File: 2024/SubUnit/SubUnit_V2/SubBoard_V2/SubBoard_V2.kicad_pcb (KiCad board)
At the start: 2 copper layers, 66.8 x 58 mm, 28 parts, among them J1 Conn_01x02_Socket, J10 Conn_01x02_Socket, J11 Conn_01x03_Socket, J12 Conn_01x02_Socket, J13 Conn_01x02_Socket, J14 Conn_01x05_Socket, J15 Conn_01x05_Socket, J16 Conn_01x02_Socket, J18 Conn_01x07_Socket, J19 Conn_01x07_Socket, J2 Conn_01x02_Socket, J3 Conn_01x02_Socket, J4 Conn_01x02_Socket, J5 Conn_01x02_Socket, J6 Conn_01x02_Socket, J7 Conn_01x02_Socket, J8 Conn_01x02_Socket, J9 Conn_01x02_Socket

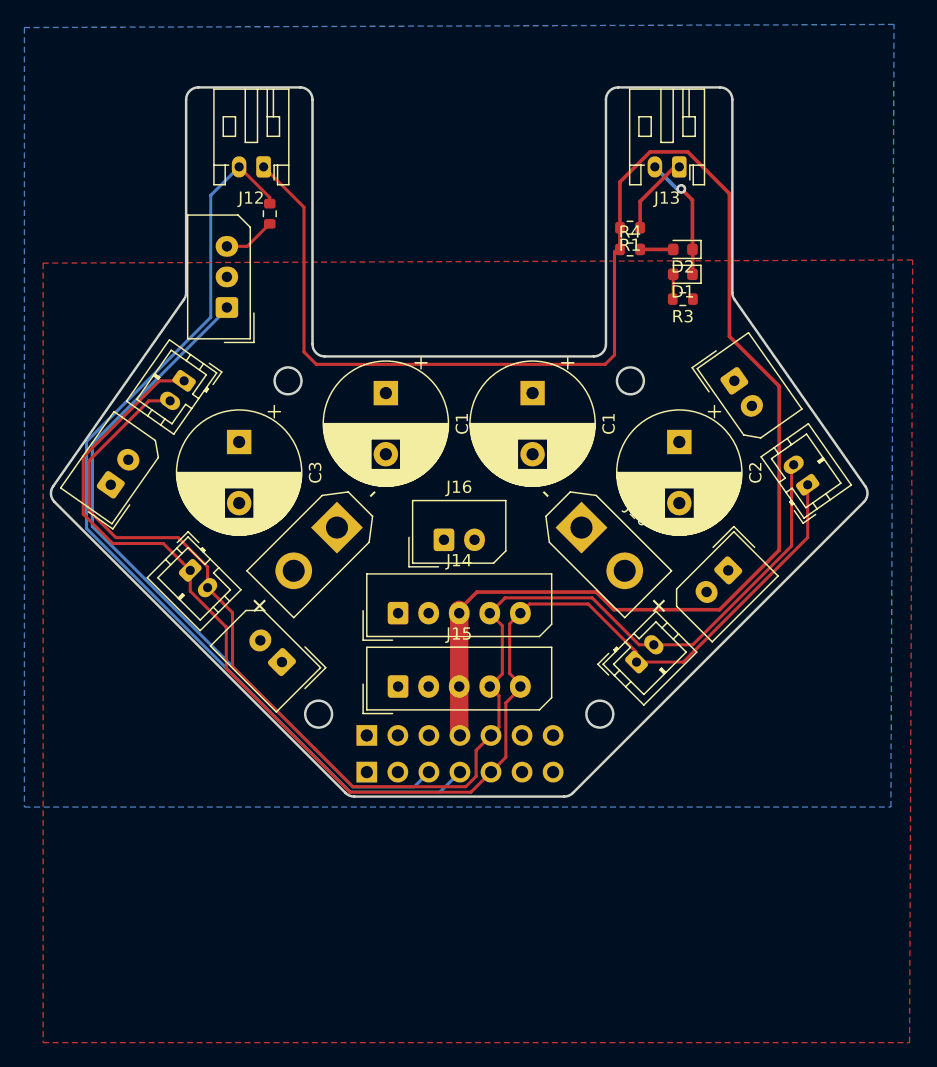
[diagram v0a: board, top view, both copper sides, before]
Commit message: 完成
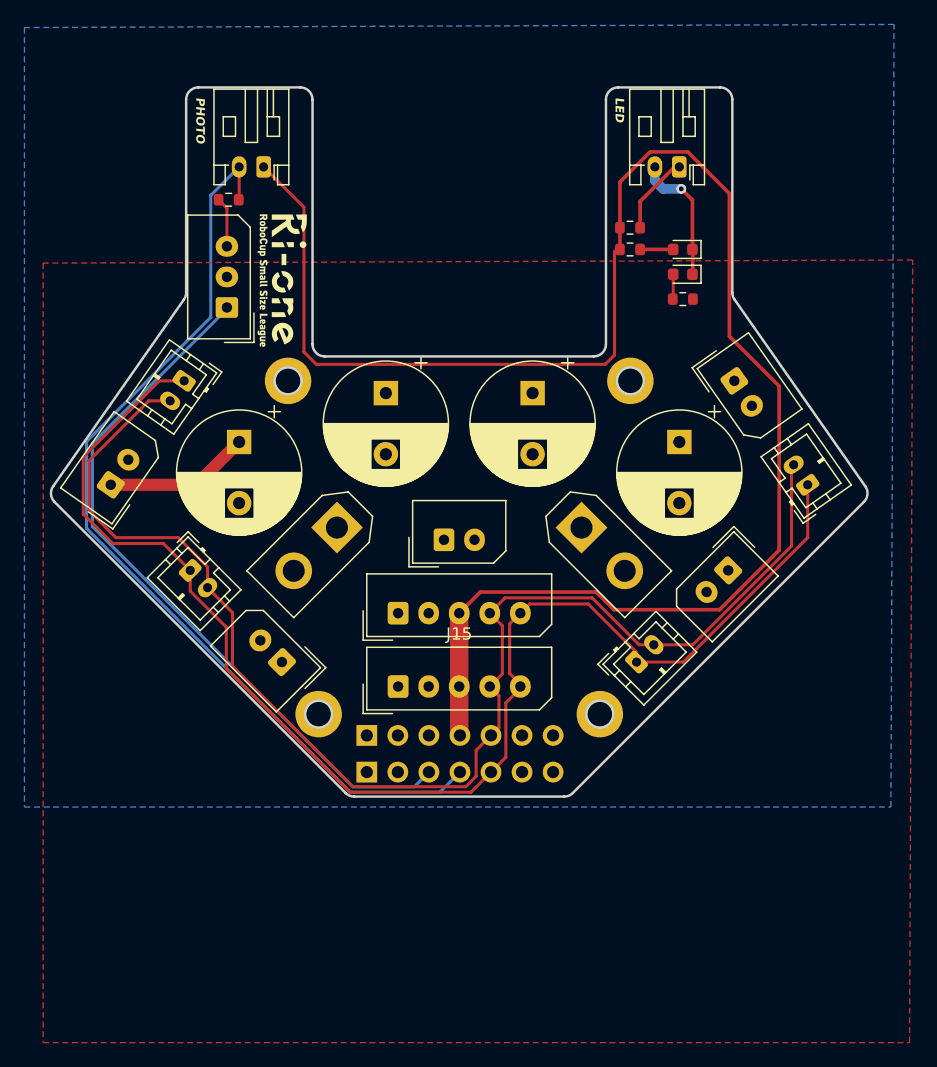
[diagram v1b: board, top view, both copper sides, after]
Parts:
- removed the C1 at (-6.00, -4.00)
- added ?: , , F.Cu at (14.0, -5.00)
- added ?: , , F.Cu at (11.6, 22.6)
- added ?: , , F.Cu at (-11.4, 22.6)
- added ?: , , F.Cu at (-14.0, -5.00)
- added C4: 1000u, Capacitor_THT:CP_Radial_D10.0mm_P5.00mm, F.Cu at (-6.00, -4.00)
- added G***: LOGO, KotaroOCHIISHI:rione22, F.Cu at (-14.5, -13.2)
- added G***: LOGO, KotaroOCHIISHI:qr11, B.Cu at (17.3, -16.5)
- added G***: LOGO, KotaroOCHIISHI:rione12, B.Cu at (0.00, 8.00)
- added G***: LOGO, KotaroOCHIISHI:black, B.Cu at (-24.0, -34.0)
- added G***: LOGO, KotaroOCHIISHI:black, B.Cu at (24.0, -34.0)
- C1, C2, C3: value 1500u -> 1000u
- moved R2 3.55 mm to (-18.9, -19.8), turned to 0 degrees
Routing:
- net +15V: track 0.00 -> 11.9 mm
- net TR_SIGNAL: track 78.9 -> 77.6 mm
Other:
- board text added: "GND +BATT +6.5V CANH CANL"
- board text added: "LED"
- board text added: "PHOTO"
- board text added: "github.com /Rione /ssl-Circuit"

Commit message: もう発注できる
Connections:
- J10 pad 1: +15V -> GNDPWR
- J10 pad 2: GNDPWR -> +15V
- J9 pad 1: +15V -> GNDPWR
- J9 pad 2: GNDPWR -> +15V
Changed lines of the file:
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@@
       (stroke (width 0.1) (type solid)) (layer "F.Fab"))
     (pad "1" thru_hole rect locked (at 0 0 225) (size 3 3) (drill 1.8) (layers "*.Cu" "*.Mask")
-      (net 1 "+15V") (pinfunction "Pin_1") (pintype "passive"))
+      (net 7 "GNDPWR") (pinfunction "Pin_1") (pintype "passive"))
     (pad "2" thru_hole circle locked (at 5 0 225) (size 3 3) (drill 1.8) (layers "*.Cu" "*.Mask")
-      (net 7 "GNDPWR") (pinfunction "Pin_2") (pintype "passive"))
+      (net 1 "+15V") (pinfunction "Pin_2") (pintype "passive"))
     (model "${KICAD6_3DMODEL_DIR}/Connector_AMASS.3dshapes/AMASS_XT30UPB-M_1x02_P5.0mm_Vertical.wrl"
       (offset (xyz 0 0 0))
@@
       (stroke (width 0.1) (type solid)) (layer "F.Fab"))
     (pad "1" thru_hole rect locked (at 0 0 315) (size 3 3) (drill 1.8) (layers "*.Cu" "*.Mask")
-      (net 1 "+15V") (pinfunction "Pin_1") (pintype "passive"))
+      (net 7 "GNDPWR") (pinfunction "Pin_1") (pintype "passive"))
     (pad "2" thru_hole circle locked (at 5 0 315) (size 3 3) (drill 1.8) (layers "*.Cu" "*.Mask")
-      (net 7 "GNDPWR") (pinfunction "Pin_2") (pintype "passive"))
+      (net 1 "+15V") (pinfunction "Pin_2") (pintype "passive"))
     (model "${KICAD6_3DMODEL_DIR}/Connector_AMASS.3dshapes/AMASS_XT30UPB-M_1x02_P5.0mm_Vertical.wrl"
       (offset (xyz 0 0 0))
